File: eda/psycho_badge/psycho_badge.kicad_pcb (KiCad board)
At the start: 2 copper layers, 152.4 x 101.6 mm, 2 parts

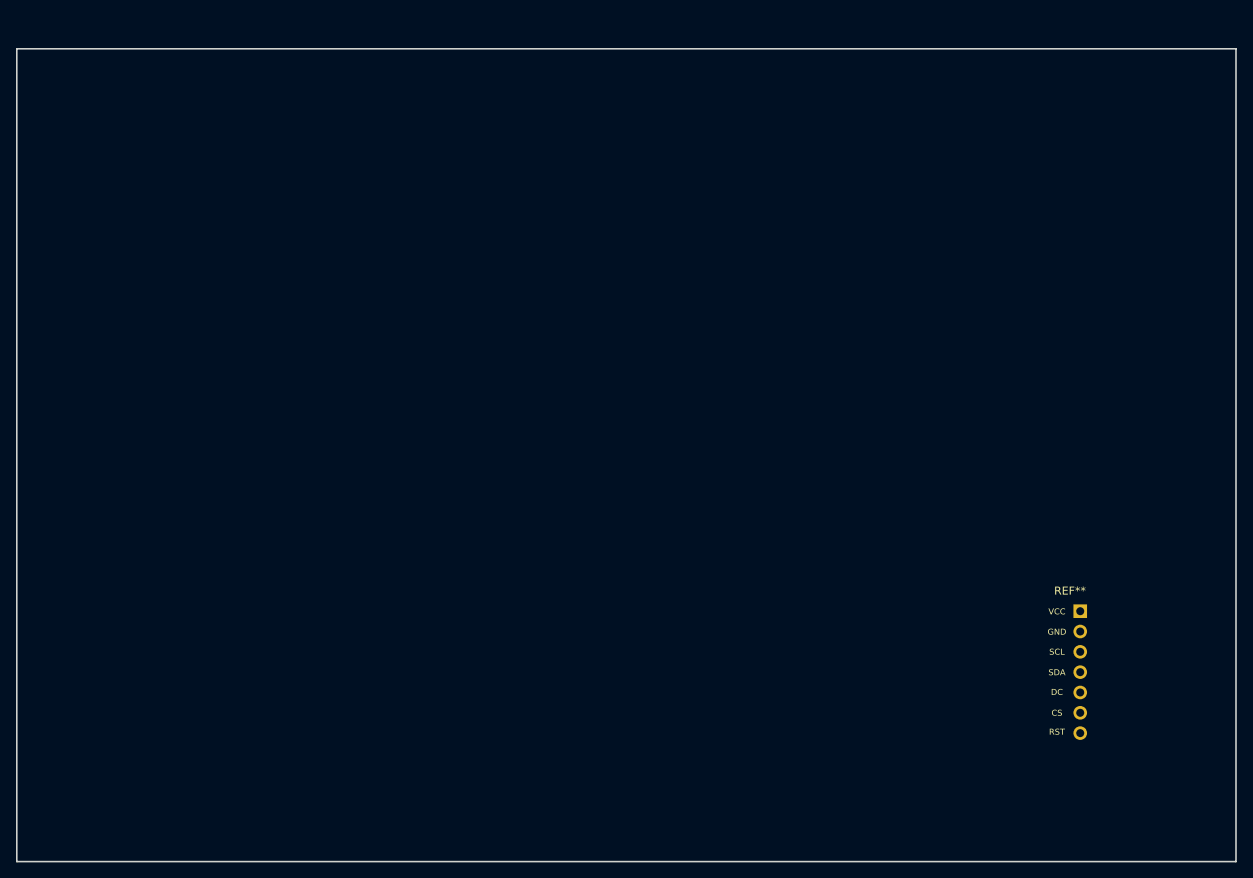
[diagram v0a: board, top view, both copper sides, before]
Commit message: pre dc33 updates
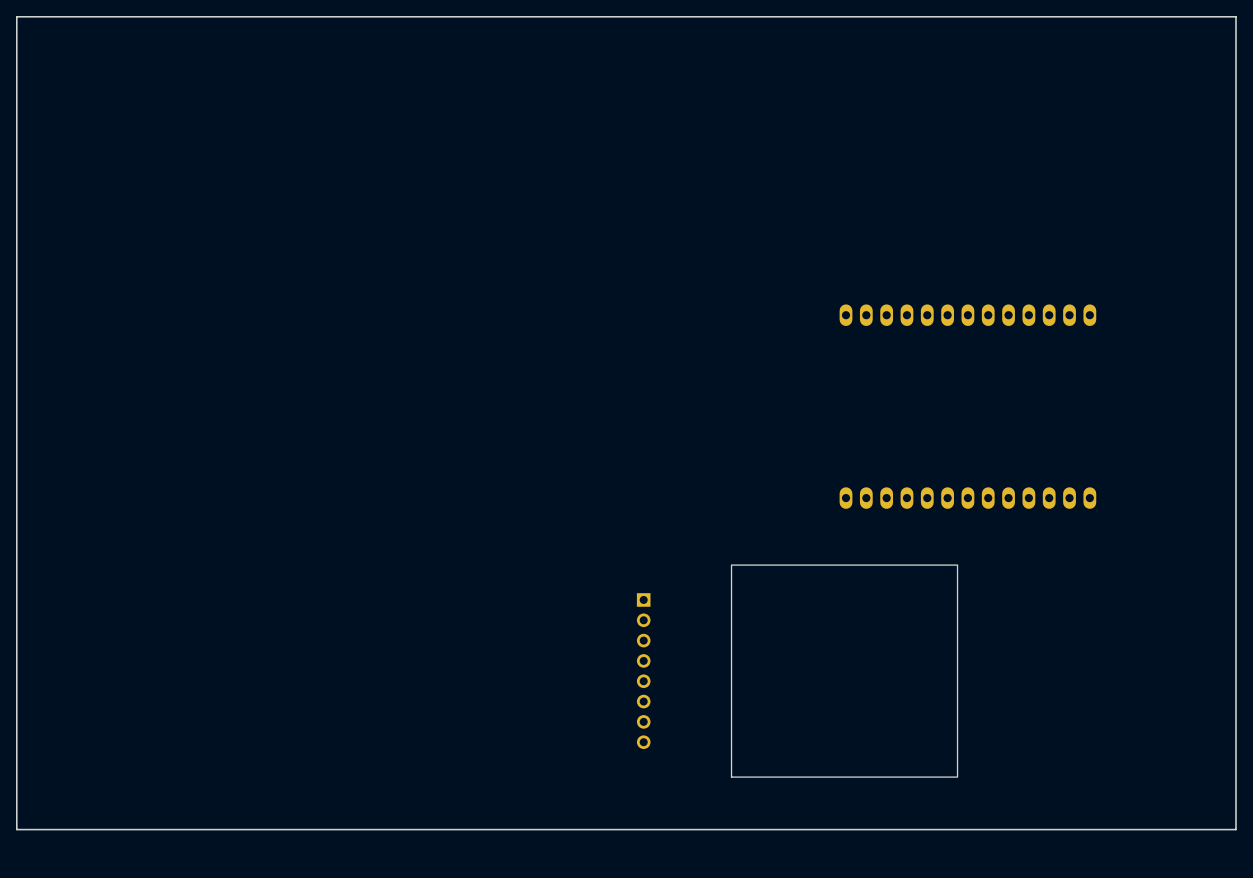
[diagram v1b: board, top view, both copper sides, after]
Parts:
- removed the REF** at (195.0, 111.0)
- added REF**: TFT_LCD_ST7735S_MSP1443_SPI_1_44IN_RearMnt, 0_local:TFT_LCD_ST7735S_MSP1443_SPI_1_44IN_RearMnt, F.Cu at (142.6, 109.5)
- added REF**: ESP32_WEMOS_LOLIN32_LITE_back, 0_local:ESP32_WEMOS_LOLIN32_LITE_back, F.Cu at (184.5, 85.6)
- moved REF** 4.00 mm to (140.5, 81.7)
